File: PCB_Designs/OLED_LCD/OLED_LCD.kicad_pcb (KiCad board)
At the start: 2 copper layers, 104.1 x 67.8 mm, 28 parts, among them P1 CONN_01X10, P2 CONN_01X16, P3 CONN_01X01, P4 CONN_01X01, P5 CONN_01X01, P6 CONN_01X01, SW1 Rotary_Encoder_Switch, U1 MCP23017, U2 MCP23017, U3 CHERRY-MX

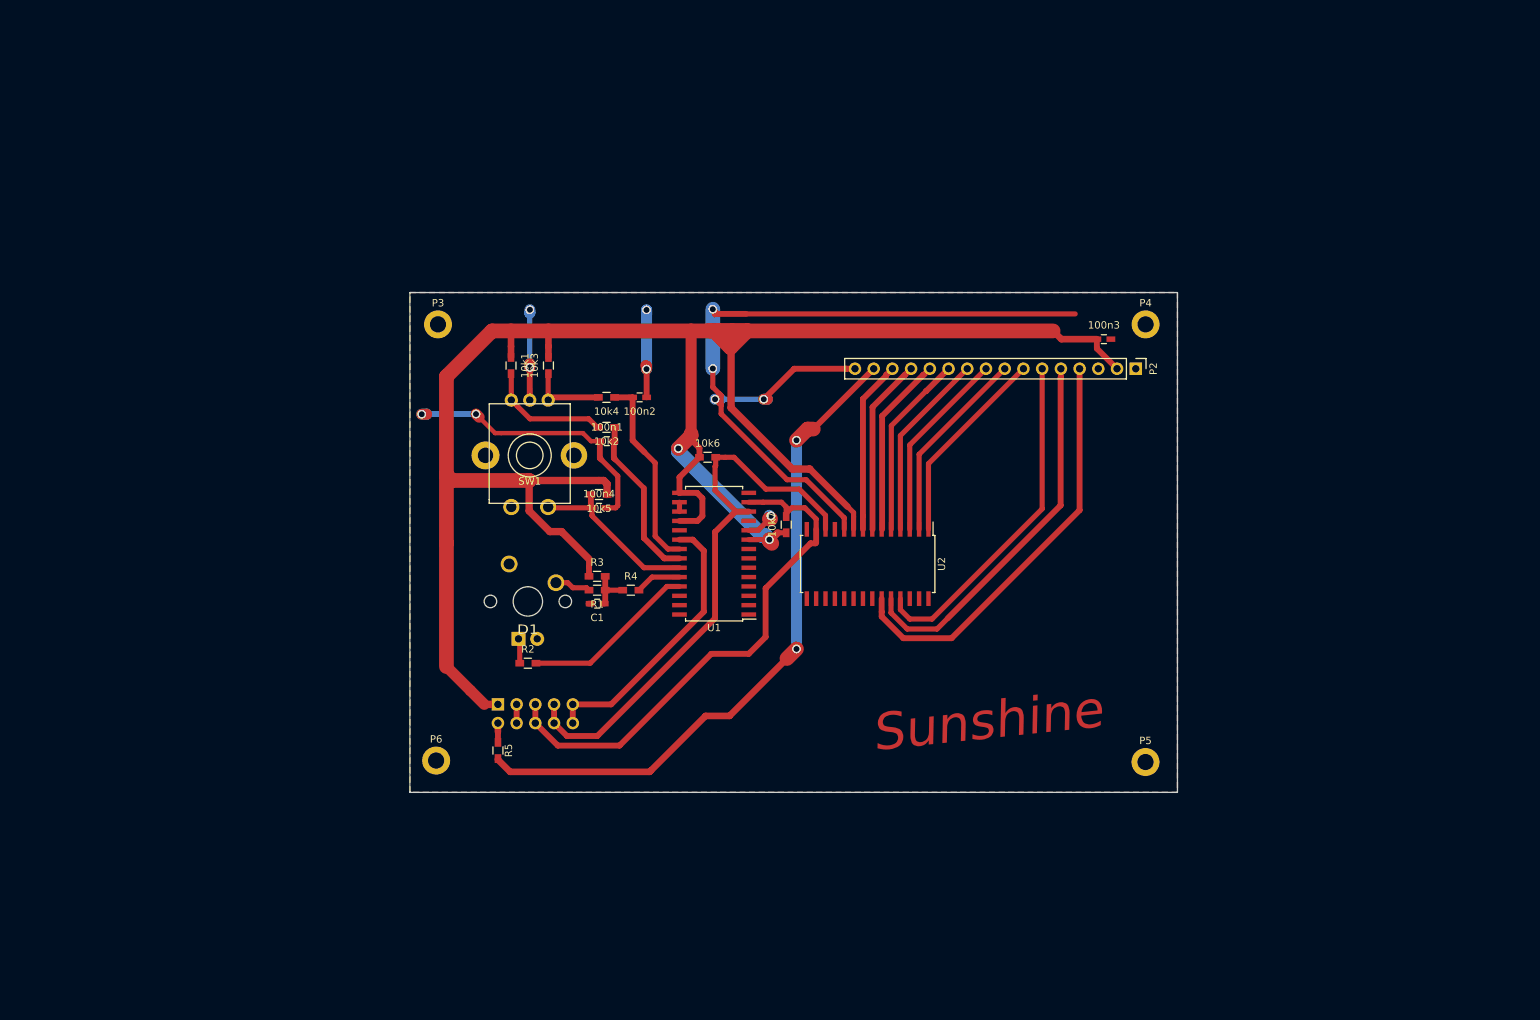
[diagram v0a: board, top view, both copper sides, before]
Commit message: Hej
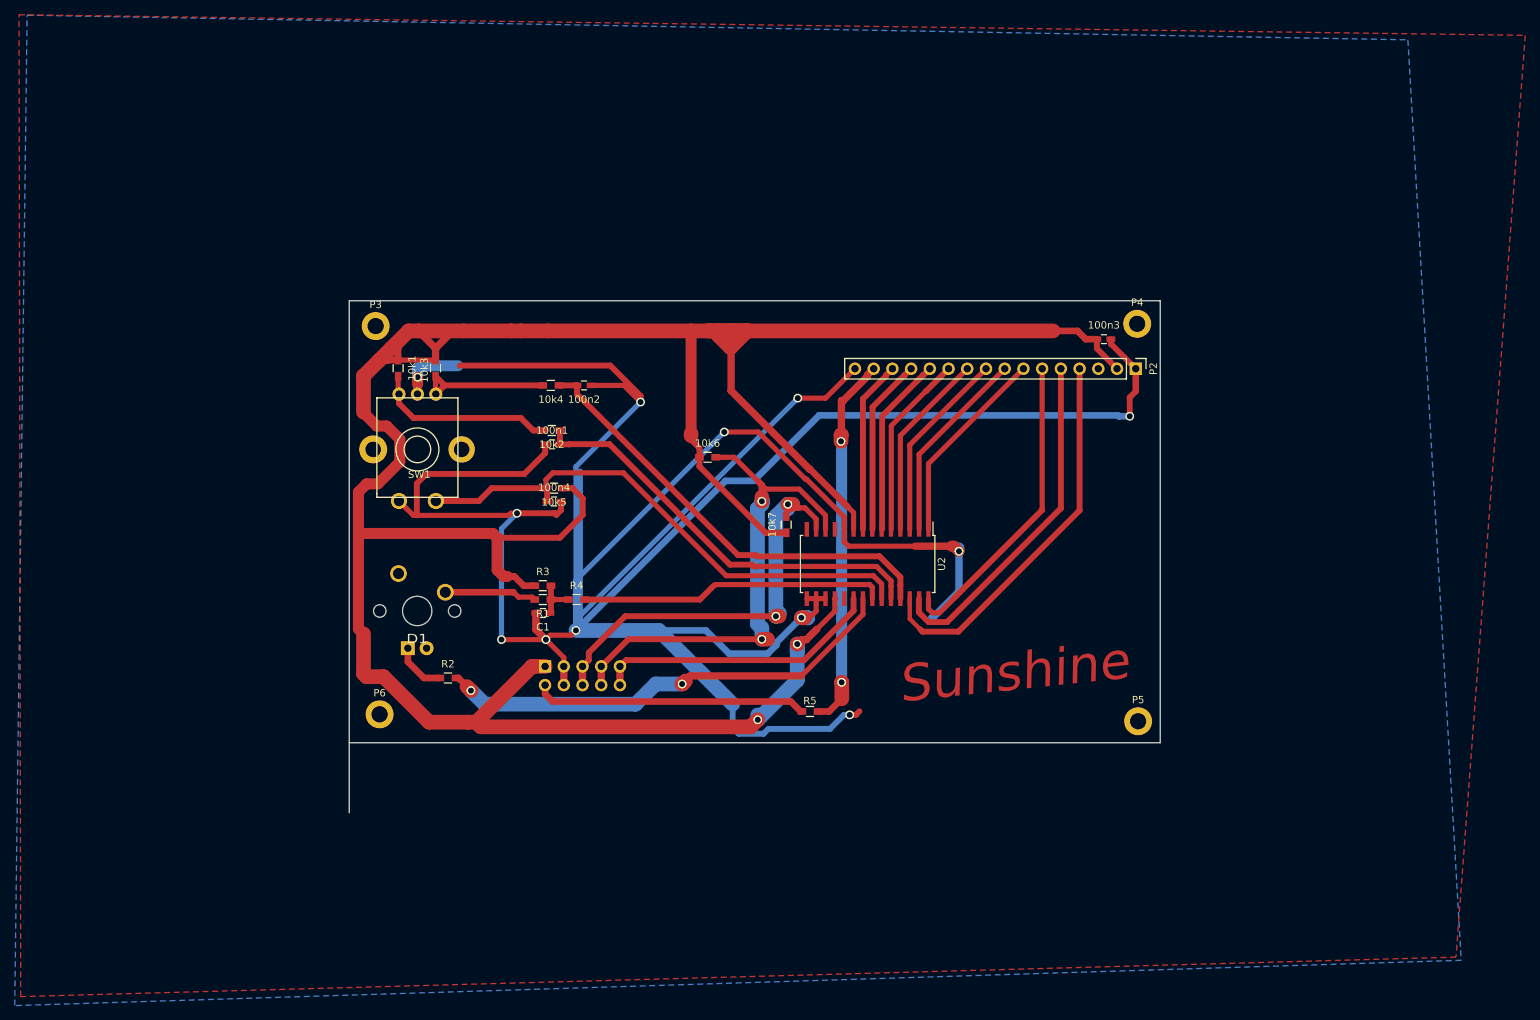
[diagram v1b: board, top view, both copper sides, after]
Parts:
- removed U1: MCP23017, Housings_SOIC:SOIC-28W_7.5x17.9mm_Pitch1.27mm
- moved R5 42.7 mm to (140.9, 134.1), turned to 0 degrees
- moved 10k1 15.3 mm to (85.0, 87.5)
- moved 10k3 15.3 mm to (90.1, 87.5)
- moved SW1 15.3 mm to (87.6, 98.5)
- moved U3 15.1 mm to (87.6, 120.4)
- moved D1 15.1 mm to (87.6, 120.4)
- moved R2 11.0 mm to (91.8, 129.5)
- moved P6 9.91 mm to (82.5, 134.4)
- moved P3 8.46 mm to (82.0, 81.8)
- moved P1 8.22 mm to (105.0, 127.9)
- moved 10k4 7.72 mm to (105.7, 89.8)
- moved 100n2 7.72 mm to (110.2, 89.8)
- moved R3 7.47 mm to (104.6, 117.0)
- moved C1 7.47 mm to (104.7, 120.7)
- moved R1 7.47 mm to (104.6, 118.9)
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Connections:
- U2 pad 18: Net-(U2-Pad18) -> /VCC5
- U2 pad 20: Net-(U2-Pad20) -> /INTA
- U2 pad 21: Net-(U2-Pad21) -> /BUTT_LED
- U2 pad 22: Net-(U2-Pad22) -> /BUTTON_2
- U2 pad 23: /RS -> /ENCODERSW
- U2 pad 24: /RW -> /ENCODERB
- U2 pad 25: /E -> /ENCODERA
- U2 pad 26: Net-(U2-Pad26) -> /RS
- U2 pad 27: Net-(U2-Pad27) -> /RW
- U2 pad 28: Net-(U2-Pad28) -> /E
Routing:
- net GND: track 190.3 -> 519.4 mm, vias 11 -> 12
- net /VCC5: track 297.7 -> 404.0 mm
- net /ENCODERSW: track 23.7 -> 72.9 mm
- net /BUTT_LED: track 23.8 -> 64.5 mm, vias 0 -> 2
- net /LCD_BACKLIGHT: track 91.1 -> 50.7 mm
- net /BUTTON_2: track 6.24 -> 41.6 mm
- net Net-(P1-Pad2): track 2.62 -> 37.0 mm
- net /ENCODERB: track 22.9 -> 57.2 mm
- net /ENCODERA: track 26.6 -> 60.8 mm
- net /SDA#: track 72.5 -> 58.5 mm, vias 0 -> 2
- net /SCL#: track 79.5 -> 69.5 mm, vias 0 -> 2
- net Net-(10k3-Pad1): track 10.6 -> 19.2 mm
- net Net-(10k1-Pad2): track 17.0 -> 24.9 mm
- net Net-(R1-Pad2): track 4.91 -> 12.6 mm
- net /E: track 46.5 -> 42.0 mm
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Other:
- board size 104.1 x 67.8 mm -> 110 x 69.5 mm
